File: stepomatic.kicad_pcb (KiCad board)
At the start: 2 copper layers, 50 x 30 mm, 87 parts, among them J1 I2C, J2 5V Switch, J4 USB_B_Micro, Q1 MMBT3904, Q2 MMBT3904, SW1 Mode, SW2 RST, U1 HDC1080DMBR, U2 SK6812, U3 ULN2003A, U4 CH340C, U5 28BYJ-48, U6 AMS1117, U7 ESP-07

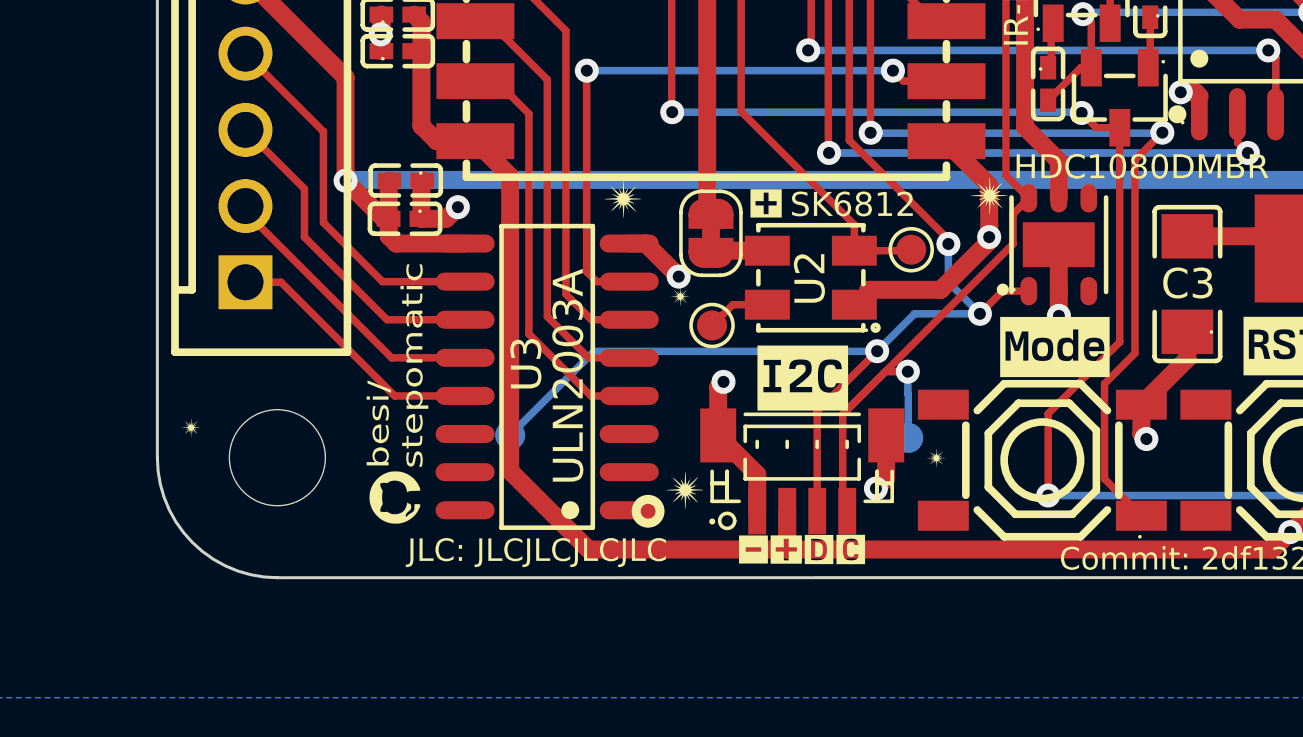
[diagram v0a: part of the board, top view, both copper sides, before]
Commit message: Add OSHW Logo
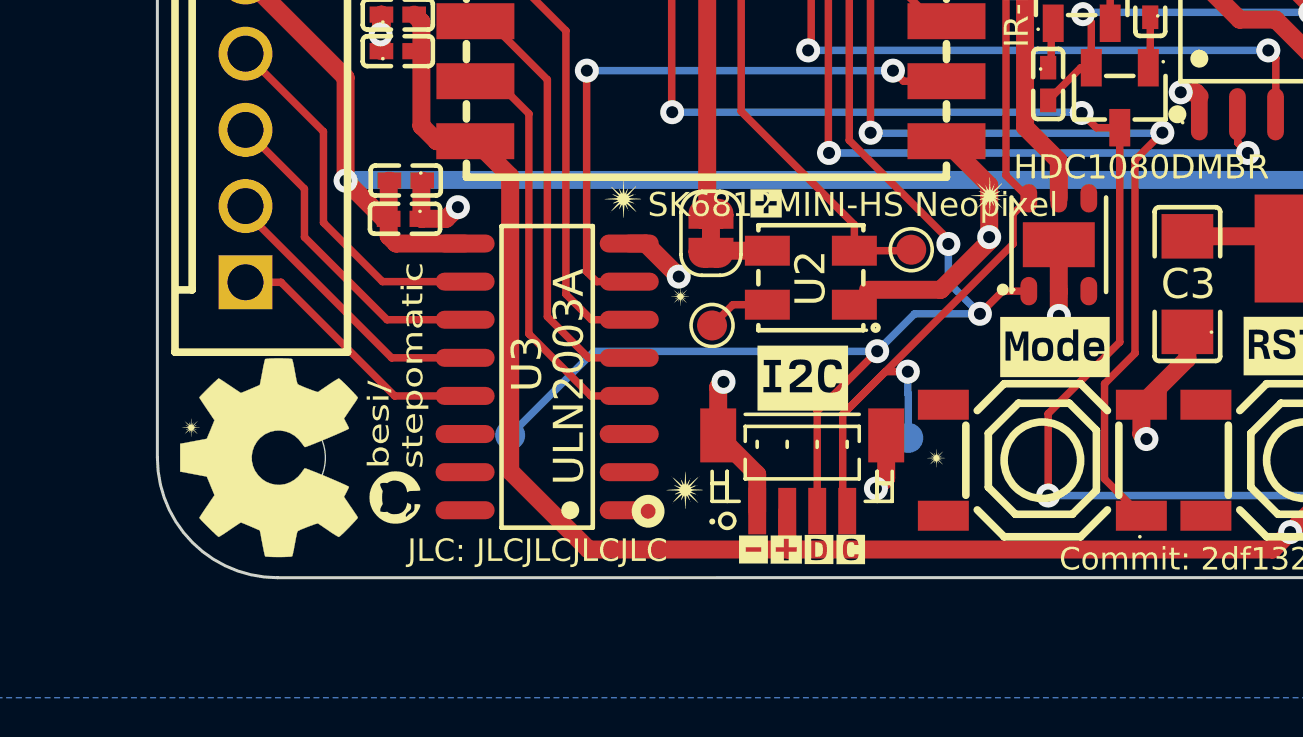
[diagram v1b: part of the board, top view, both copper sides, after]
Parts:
- added OSHW1: Logo_Open_Hardware_Small, Symbol:OSHW-Symbol_6.7x6mm_SilkScreen, F.Cu at (103.7, 96.0)
- U2: value SK6812 -> SK6812MINI-HS Neopixel
